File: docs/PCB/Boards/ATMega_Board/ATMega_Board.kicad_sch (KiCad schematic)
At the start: 22 parts, among them J1 Conn_02x10_Odd_Even, J2 AVR-ISP-10, J3 Conn_01x10_Pin, J4 Conn_01x10_Pin, SW1 Tact Switch 6x6mm / 13mm, U1 ATmega328PB-A, U2 ATmega328P-P, Y1 Crystal

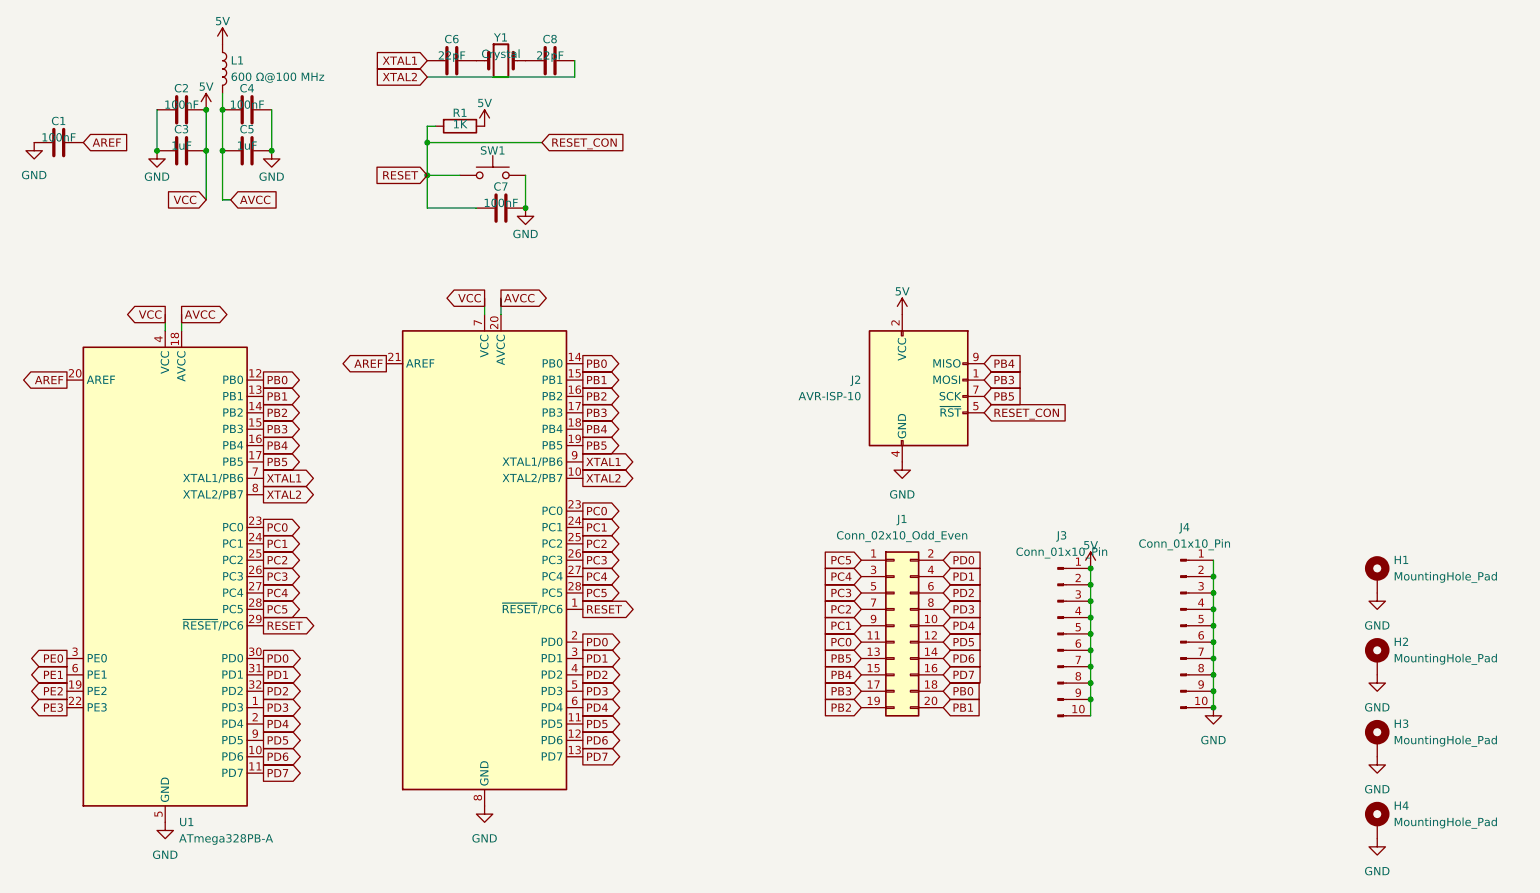
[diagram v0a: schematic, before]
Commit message: Hardware docs updated.
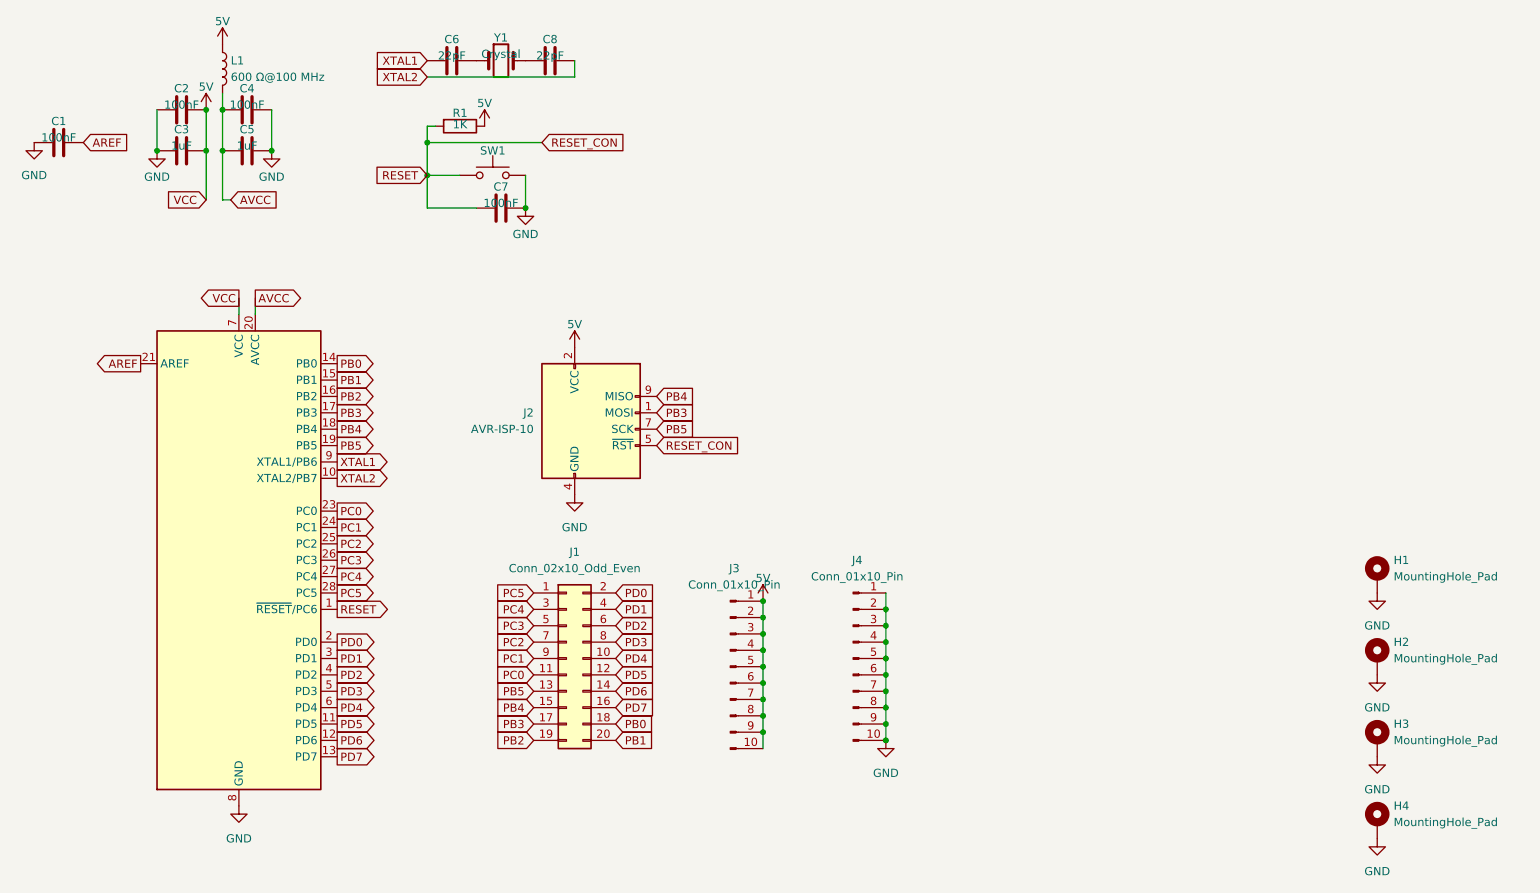
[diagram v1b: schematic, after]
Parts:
- removed U1: ATmega328PB-A, Package_QFP:TQFP-32_7x7mm_P0.8mm, symbol MCU_Microchip_ATmega:ATmega328PB-A
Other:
- moved on the sheet: J1, J2, J3, J4
